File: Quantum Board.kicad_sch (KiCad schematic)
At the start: 129 parts, among them U1 Raspberry_Pi_Pico

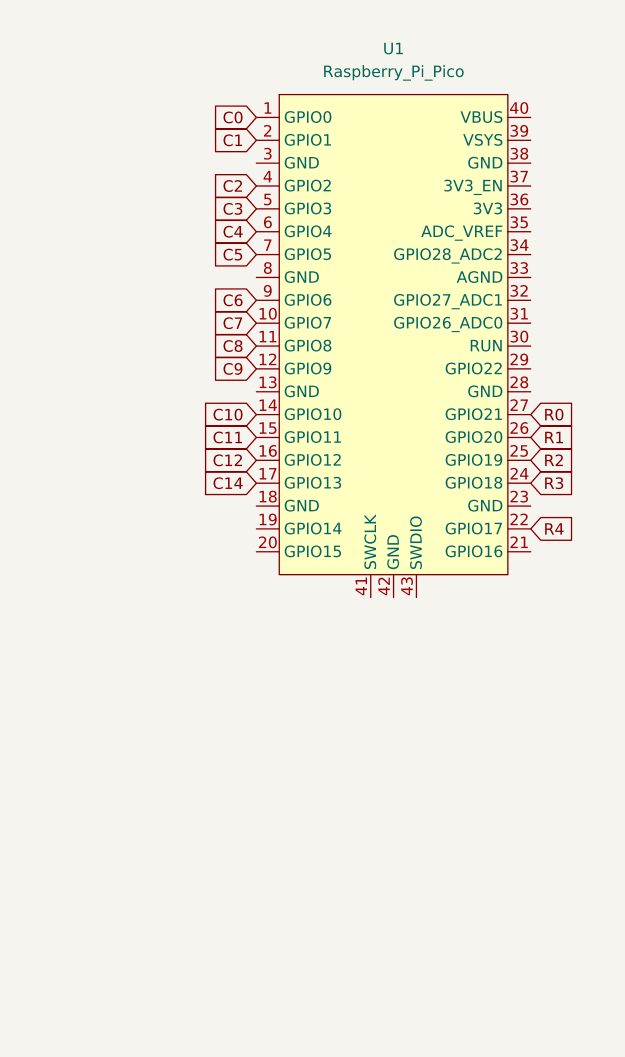
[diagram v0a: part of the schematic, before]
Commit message: Quantum Board Part 3
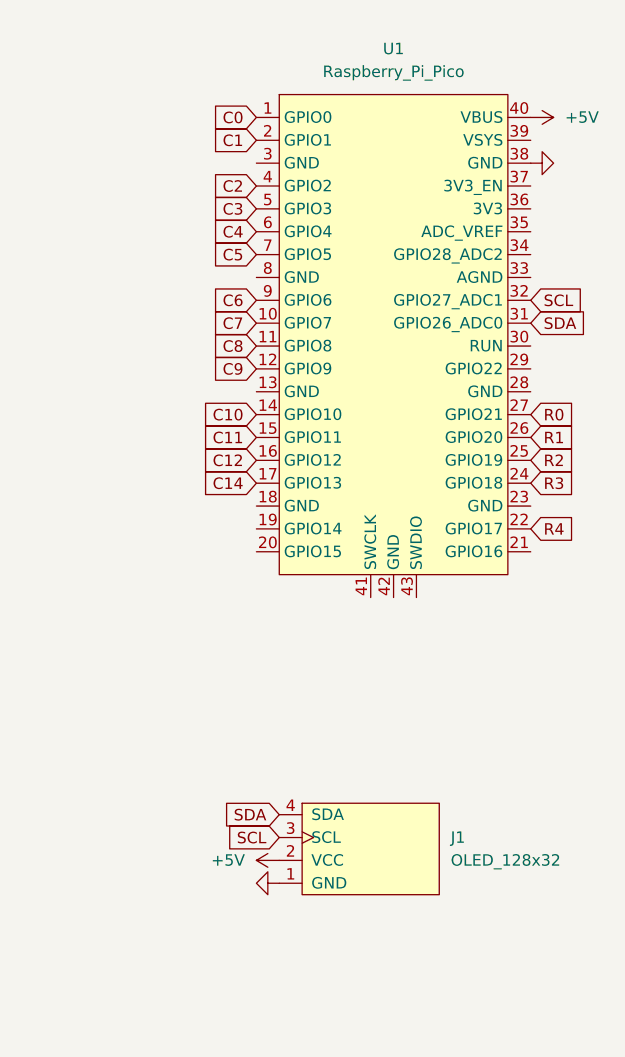
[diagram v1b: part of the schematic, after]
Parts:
- added J1: OLED_128x32, ScottoKeebs_Components:OLED_128x32, symbol ScottoKeebs:OLED_128x32
- D1, D10, D11, D12, D13, D14, D15, D16, D17, D18, D19, D2, D20, D21, D22, D23, D24, D25, D26, D27, D28, D29, D3, D30, D31, D32, D33, D34, D35, D36, D37, D38, D39, D4, D40, D41, D42, D43, D44, D45, D46, D47, D48, D49, D5, D50, D51, D52, D53, D54, D55, D56, D57, D58, D59, D6, D63, D67, D68, D69, D7, D70, D8, D9: footprint (none) -> ScottoKeebs_Components:Diode_DO-35
- S1, S14, S15, S28, S29, S42, S43, S56, S57, S58, S59, S61: footprint (none) -> ScottoKeebs_Choc:Choc_V1_1.50u
- S10, S11, S12, S13, S16, S17, S18, S19, S2, S20, S21, S22, S23, S24, S25, S26, S27, S3, S30, S31, S32, S33, S34, S35, S36, S37, S38, S39, S4, S40, S41, S44, S45, S46, S47, S48, S49, S5, S50, S51, S52, S53, S54, S55, S6, S62, S63, S64, S7, S8, S9: footprint (none) -> ScottoKeebs_Choc:Choc_V1_1.00u
- S60: footprint (none) -> ScottoKeebs_Choc:Choc_V1_5.50u
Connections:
- net SDA: now reaches U1.31 (GPIO26_ADC0)
- net SDA: now also J1.4 (SDA)
- net SCL: now reaches U1.32 (GPIO27_ADC1)
- net SCL: now also J1.3 (SCL)
- net GND: now reaches U1.38 (GND)
- net GND: now also J1.1 (GND)
- net +5V: now reaches U1.40 (VBUS)
- net +5V: now also J1.2 (VCC)

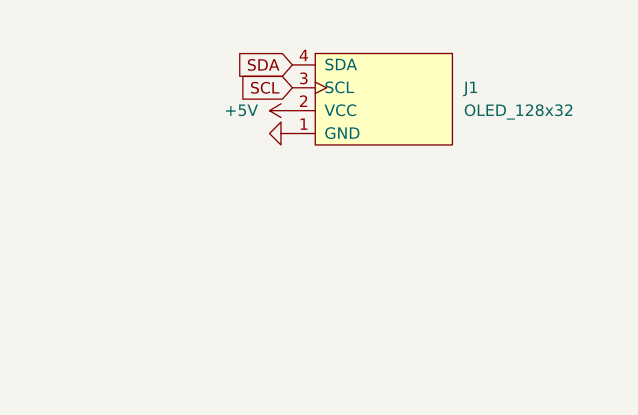
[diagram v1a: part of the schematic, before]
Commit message: Quantum Board Part 5
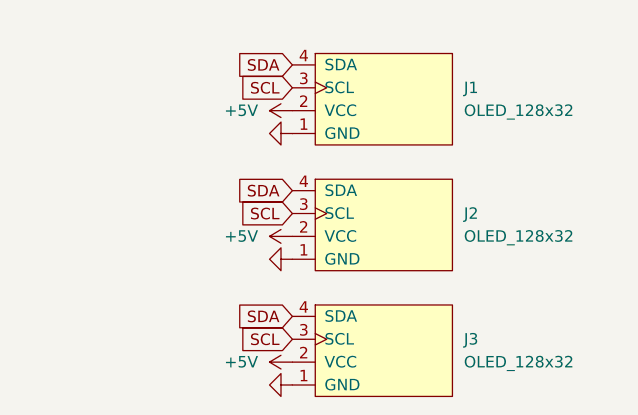
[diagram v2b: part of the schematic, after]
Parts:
- added J2, J3: OLED_128x32, ScottoKeebs_Components:OLED_128x32, symbol ScottoKeebs:OLED_128x32
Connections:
- net +5V: now also J2.2 (VCC), J3.2 (VCC)
- net GND: now also J2.1 (GND), J3.1 (GND)
- net SCL: now also J2.3 (SCL), J3.3 (SCL)
- net SDA: now also J2.4 (SDA), J3.4 (SDA)
